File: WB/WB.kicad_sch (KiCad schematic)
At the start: 43 parts, among them J1 Conn_01x04, J2 Conn_01x04, J3 Conn_01x04, J4 Conn_01x04, J5 Pump, J6 Actuator, J7 Actuator, J8 Screw_Terminal_01x02, M1 Fan, Q1 Q_NMOS_GDS, Q2 Q_NMOS_GDS, Q3 Q_NMOS_GDS, Q4 Q_NMOS_GDS, Q5 Q_NMOS_GDS, Q6 Q_NMOS_GDS, Q7 Q_NMOS_GDS, Q8 Q_NPN_ECB, SW1 SW_Push, SW2 SW_Push, SW3 SW_Push, SW4 SW_Push, SW5 SW_Push, SW6 SW_Push, U1 74HC165, U2 74HC595, U3 TB6643KQ, U4 Arduino_Micro

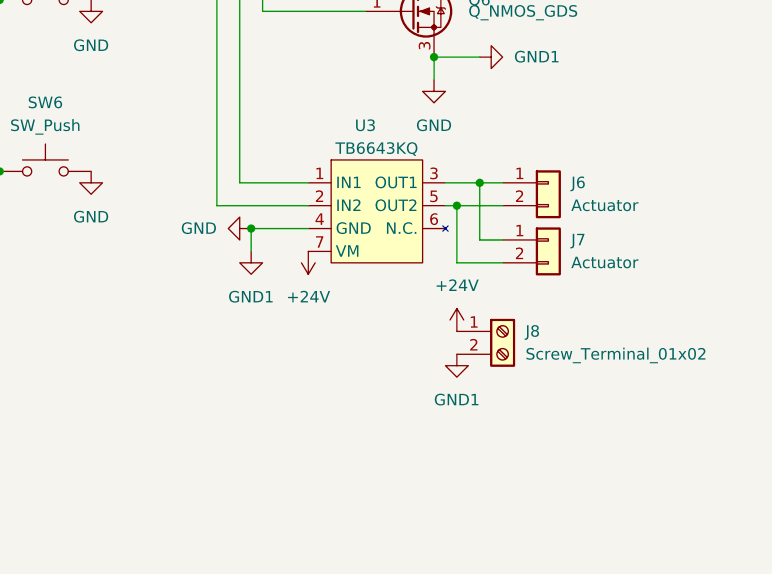
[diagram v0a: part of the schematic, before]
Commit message: 回路図の修正
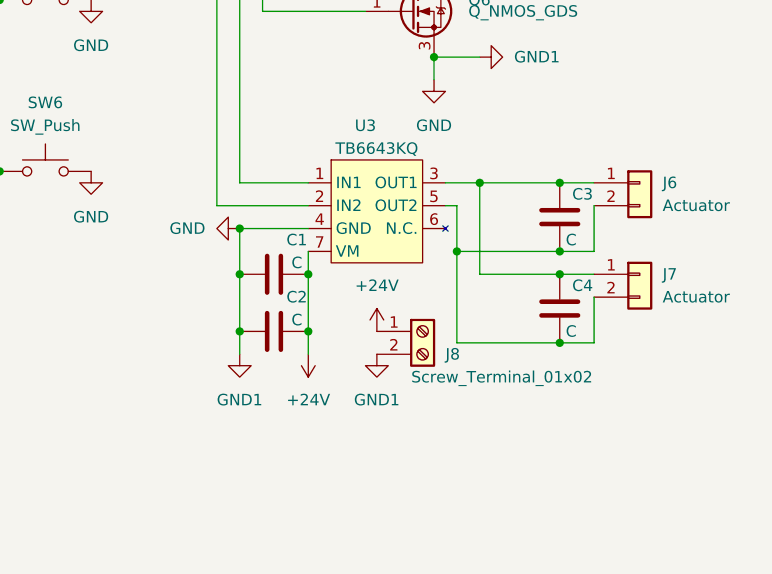
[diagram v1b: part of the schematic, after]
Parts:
- added C1, C3, C4: C, Capacitor_THT:C_Rect_L4.0mm_W2.5mm_P2.50mm, symbol Device:C
- added C2: C, Capacitor_THT:C_Radial_D8.0mm_H11.5mm_P3.50mm, symbol Device:C
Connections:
- net +24V: now also C1.2, C2.2
- net GND: now also C1.1, C2.1
- net at J6.1 (Pin_1), J7.1 (Pin_1), U3.3 (OUT1): now also C3.1, C4.1
- net at J6.2 (Pin_2), J7.2 (Pin_2), U3.5 (OUT2): now also C3.2, C4.2
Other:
- moved on the sheet: J6, J7, J8
